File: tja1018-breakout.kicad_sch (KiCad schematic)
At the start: 13 parts, among them J101 Conn_01x03_Pin, J102 Conn_01x05, J103 Conn_01x05, U101 TJA1028

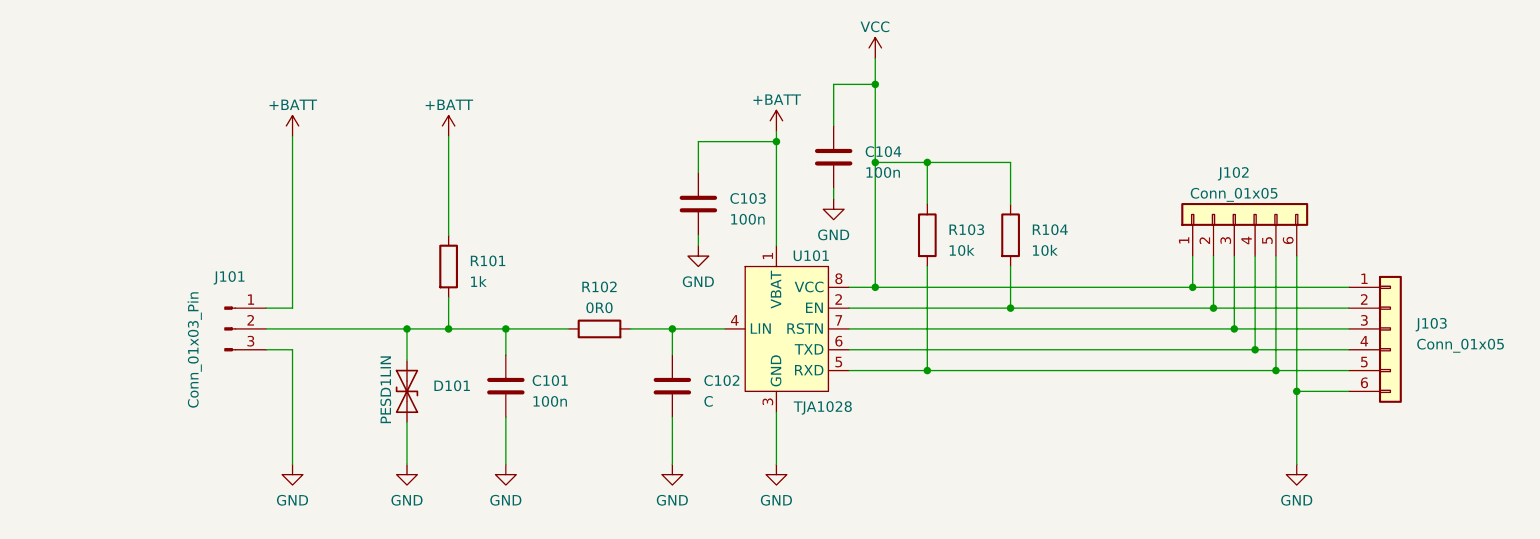
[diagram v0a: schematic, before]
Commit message: add readme
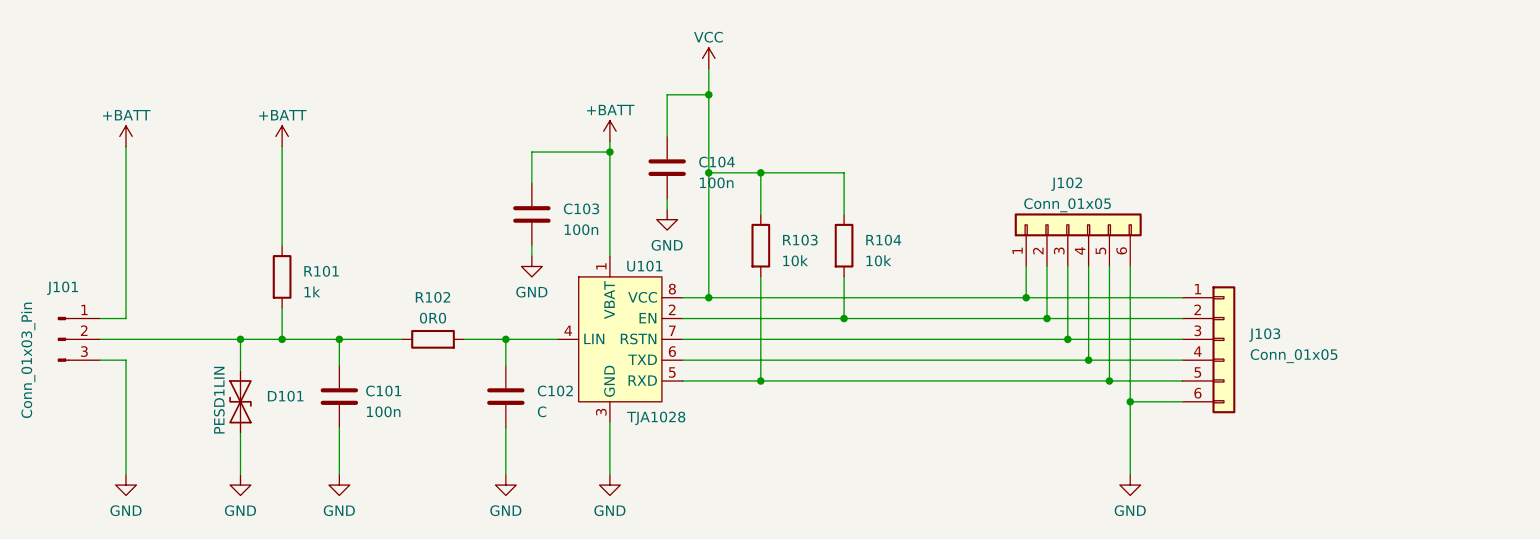
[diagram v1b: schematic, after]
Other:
- title: (none) -> TJA1028 Breakout Board
- moved on the sheet: C101, C102, C103, C104, D101, J101, J102, J103, R101, R102, R103, R104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
